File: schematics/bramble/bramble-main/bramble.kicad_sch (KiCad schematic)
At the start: 18 parts, among them Q1 DMN3300U, Q2 FDN360P, U1 Opamp_Quad

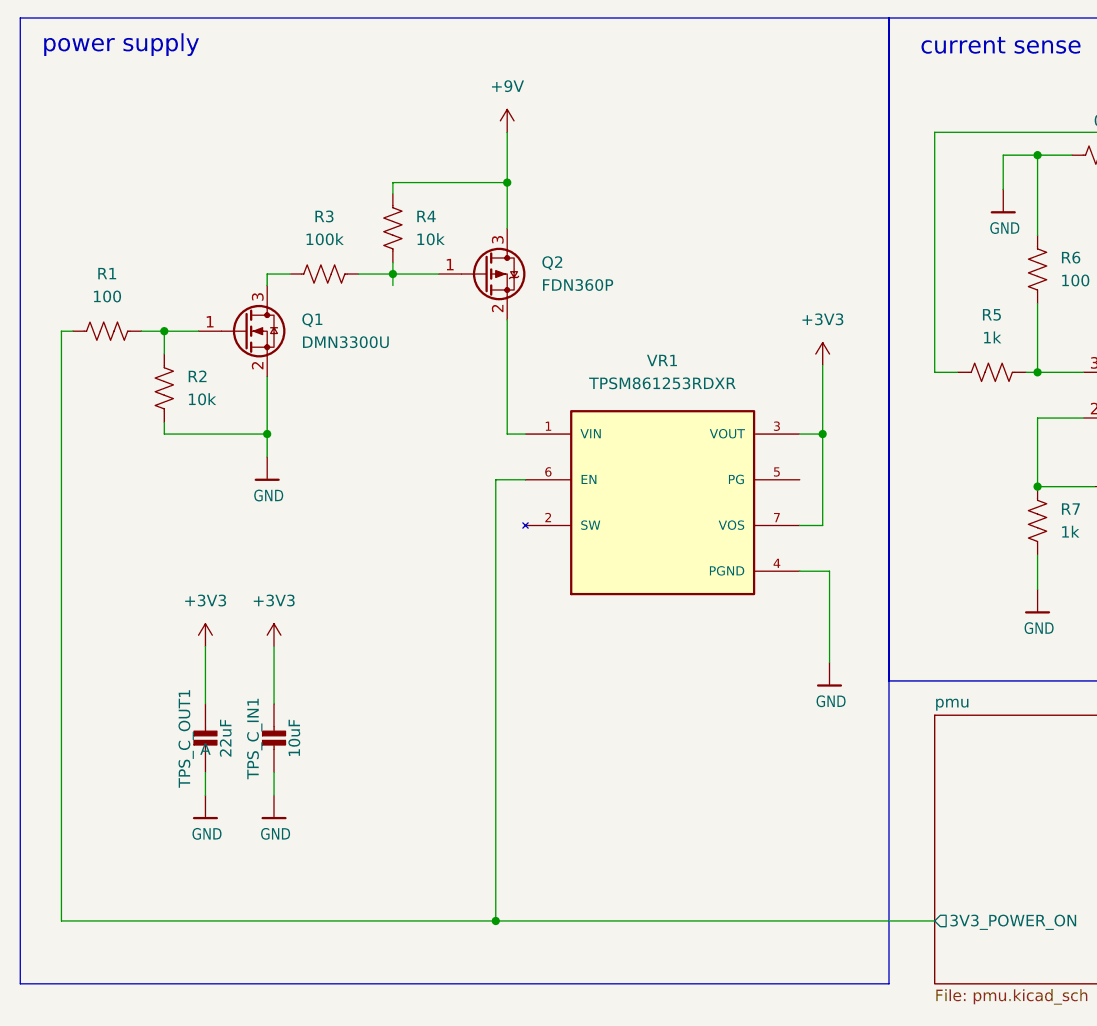
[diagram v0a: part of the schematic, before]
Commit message: Remove mosfet switching from design: new dcdc is fine alone
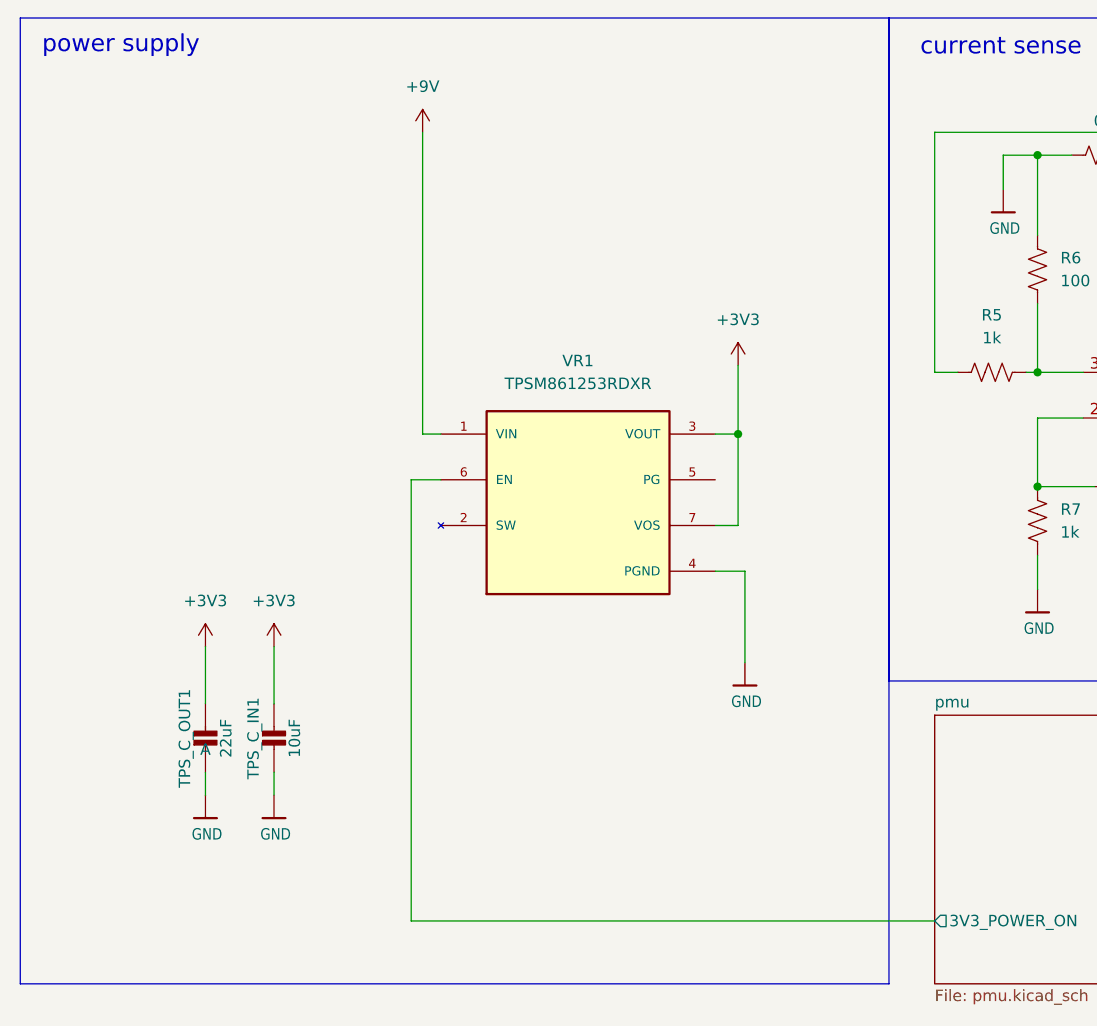
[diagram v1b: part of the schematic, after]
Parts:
- removed Q1: DMN3300U, Package_TO_SOT_SMD:SOT-23, symbol Transistor_FET:DMN3300U
- removed Q2: FDN360P, Package_TO_SOT_SMD:SOT-23, symbol Transistor_FET:FDN340P
- removed R1: 100, Resistor_SMD:R_0805_2012Metric, symbol Device:R_US
- removed R2: 10k, Resistor_SMD:R_0805_2012Metric, symbol Device:R_US
- removed R3: 100k, Capacitor_SMD:C_0805_2012Metric, symbol Device:R_US
- removed R4: 10k, Capacitor_SMD:C_0805_2012Metric, symbol Device:R_US
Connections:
- net +9V: now also VR1.1 (VIN)
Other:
- moved on the sheet: VR1
